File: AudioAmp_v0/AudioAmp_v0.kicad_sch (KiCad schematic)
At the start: 2 parts, among them J1 Conn_01x02_Pin, U1 MAU108

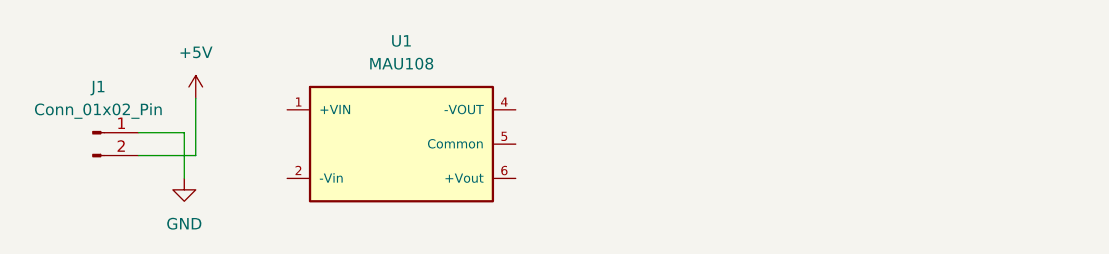
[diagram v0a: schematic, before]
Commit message: 電源回路完成
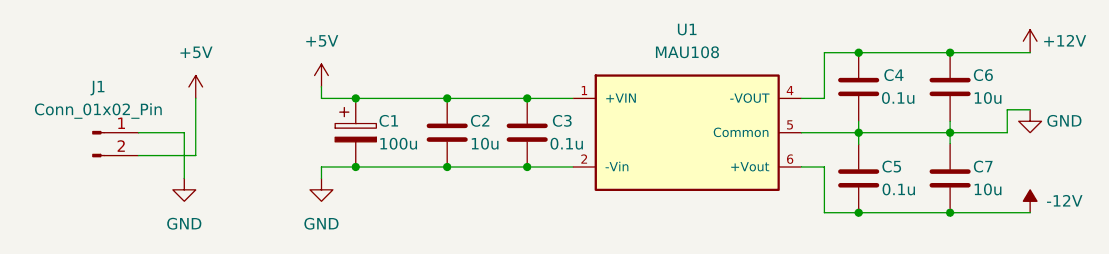
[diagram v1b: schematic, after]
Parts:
- added C1: 100u, symbol Device:C_Polarized
- added C2, C6, C7: 10u, Capacitor_SMD:C_0805_2012Metric, symbol Device:C
- added C3, C4, C5: 0.1u, Capacitor_SMD:C_0603_1608Metric, symbol Device:C
- J1: footprint (none) -> Connector_Molex:Molex_SPOX_5268-02A_1x02_P2.50mm_Horizontal
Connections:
- net +5V: now also U1.1 (+VIN), C1.1, C2.1, C3.1
- net GND: now also U1.2 (-Vin), U1.5 (Common), C1.2, C2.2, C3.2, C4.2, C5.1, C6.2, C7.1
- net +12V: now reaches U1.4 (-VOUT)
- net +12V: now also C4.1, C6.1
- net -12V: now reaches U1.6 (+Vout)
- net -12V: now also C5.2, C7.2
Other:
- moved on the sheet: U1
